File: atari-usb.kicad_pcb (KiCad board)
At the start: 2 copper layers, 30.5 x 17.8 mm, 39 parts, among them J1 USB_A, J2 DB9_Male, U1 ATmega32U4-AU, U2 TPD2EUSB30

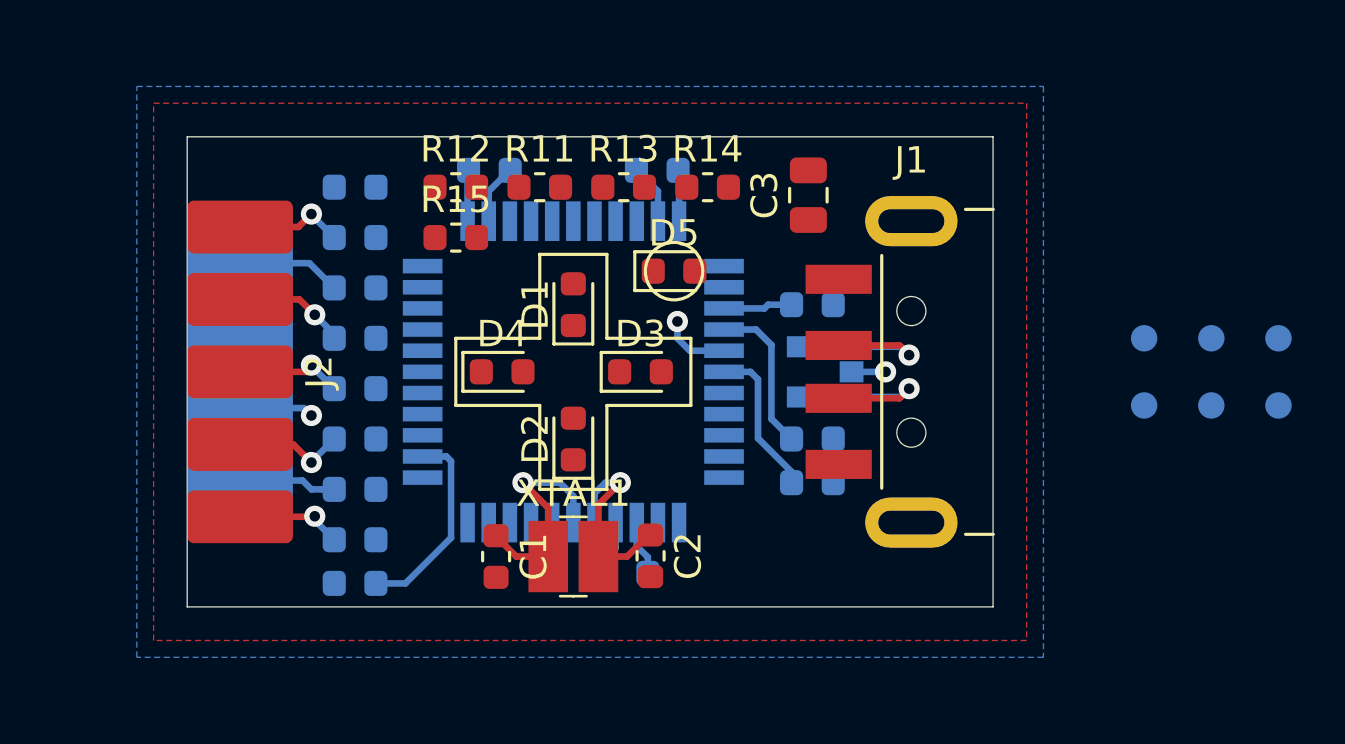
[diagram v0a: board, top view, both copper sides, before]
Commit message: Revision 0 done
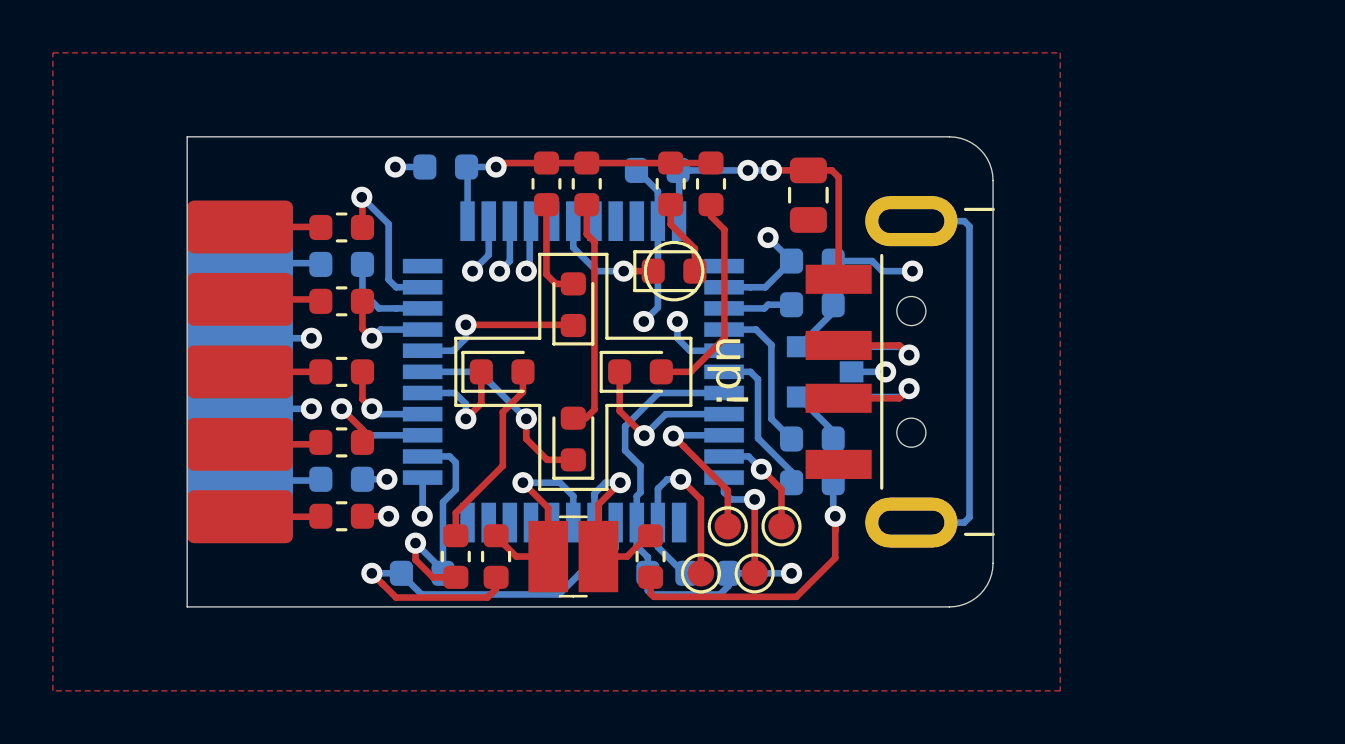
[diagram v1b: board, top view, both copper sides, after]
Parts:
- removed TP2, TP6: TestPoint, TestPoint:TestPoint_Pad_D1.0mm
- added C9: 0.1u, Capacitor_SMD:C_0603_1608Metric, B.Cu at (145.6, 80.3)
- R10, R4, R6, R7, R8: moved to F.Cu
- TP1: value TestPoint -> MISO; moved to F.Cu
- TP3: value TestPoint -> SCK; moved to F.Cu
- TP4: value TestPoint -> MOSI; moved to F.Cu
- TP5: value TestPoint -> ~RST; moved to F.Cu
- moved TP4 20.1 mm to (144.4, 90.3)
- moved R3 19.8 mm to (141.6, 92.1), turned to 180 degrees
- moved TP3 19.6 mm to (142.4, 90.3)
- moved TP5 17.9 mm to (141.4, 92.1)
- moved TP1 17.2 mm to (143.4, 92.1)
- moved R14 16.9 mm to (132.1, 91.4), turned to 90 degrees
- moved R15 8.38 mm to (140.2, 77.3), turned to 270 degrees
- moved R12 4.95 mm to (137.0, 77.3), turned to 270 degrees
- moved R13 3.30 mm to (141.7, 77.3), turned to 270 degrees
- moved C5 2.57 mm to (130.8, 92.1)
- moved C6 1.66 mm to (131.7, 76.7), turned to 0 degrees
- moved R8 1.49 mm to (127.8, 81.8)
- moved R4 1.02 mm to (127.8, 89.9)
- moved R9 1.02 mm to (127.8, 80.4)
- moved R7 0.81 mm to (127.8, 84.5)
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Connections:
- D5 pad 1: Net-(D5-Pad1) -> LED-Down
- J2 pad 7: +5V -> VBUS
- R11 pad 1: +5V -> VBUS
- R12 pad 1: +5V -> VBUS
- R13 pad 1: +5V -> VBUS
- R14 pad 1: +5V -> VBUS
- R15 pad 1: +5V -> VBUS
- R3 pad 1: +5V -> VBUS
- TP5 pad 1: Net-(TP5-Pad1) -> Net-(R3-Pad2)
- U1 pad 1: Net-(U1-Pad1) -> (no net)
- U1 pad 10: Net-(U1-Pad10) -> Net-(TP4-Pad1)
- U1 pad 11: Net-(U1-Pad11) -> Net-(TP1-Pad1)
- U1 pad 12: Net-(U1-Pad12) -> (no net)
- U1 pad 18: Net-(U1-Pad18) -> (no net)
- U1 pad 19: Net-(U1-Pad19) -> (no net)
- U1 pad 20: Net-(U1-Pad20) -> (no net)
- U1 pad 21: Net-(U1-Pad21) -> (no net)
- U1 pad 22: Net-(U1-Pad22) -> (no net)
- U1 pad 25: Net-(U1-Pad25) -> Net-(R6-Pad2)
- U1 pad 26: Net-(U1-Pad26) -> Net-(R7-Pad2)
- U1 pad 27: Net-(U1-Pad27) -> Net-(D4-Pad1)
- U1 pad 28: Net-(U1-Pad28) -> Net-(D2-Pad1)
- U1 pad 29: Net-(U1-Pad29) -> Net-(D1-Pad1)
- U1 pad 30: Net-(U1-Pad30) -> Net-(R8-Pad2)
- U1 pad 31: Net-(U1-Pad31) -> Net-(R9-Pad2)
- U1 pad 32: Net-(U1-Pad32) -> Net-(R10-Pad2)
- U1 pad 33: Net-(U1-Pad33) -> (no net)
- U1 pad 36: Net-(U1-Pad36) -> Net-(R5-Pad2)
- U1 pad 37: Net-(D5-Pad1) -> Net-(R4-Pad2)
- U1 pad 38: Net-(D4-Pad1) -> (no net)
- U1 pad 39: Net-(D3-Pad1) -> LED-Down
- U1 pad 40: Net-(D2-Pad1) -> (no net)
- U1 pad 41: Net-(D1-Pad1) -> (no net)
- U1 pad 42: Net-(U1-Pad42) -> (no net)
- U1 pad 8: Net-(U1-Pad8) -> Net-(D3-Pad1)
- U1 pad 9: Net-(U1-Pad9) -> Net-(TP3-Pad1)
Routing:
- net VBUS: track 13.6 -> 57.3 mm, vias 0 -> 7
- net GND: track 13.3 -> 49.7 mm, vias 3 -> 10
- net Net-(J1-Pad5): track 0.00 -> 15.6 mm
- net Net-(R4-Pad2): track 0.00 -> 14.4 mm, vias 0 -> 2
- net Net-(R5-Pad2): track 0.00 -> 12.6 mm, vias 0 -> 2
- net Net-(D2-Pad2): track 0.00 -> 8.78 mm
- net Net-(R3-Pad2): track 0.00 -> 8.60 mm, vias 0 -> 1
- net Net-(D3-Pad2): track 0.00 -> 8.18 mm
- net Net-(D2-Pad1): track 0.00 -> 7.52 mm, vias 0 -> 1
- net Net-(D4-Pad2): track 0.00 -> 7.25 mm
- net Net-(D1-Pad1): track 0.00 -> 6.41 mm, vias 0 -> 1
- net Net-(TP3-Pad1): track 0.00 -> 6.19 mm, vias 0 -> 1
- net Net-(D3-Pad1): track 0.00 -> 6.15 mm, vias 0 -> 1
- net Net-(R10-Pad2): track 0.00 -> 6.10 mm, vias 0 -> 1
- net Net-(R6-Pad2): track 0.00 -> 5.07 mm, vias 0 -> 1
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- added copper zone on In1.Cu, net GND
- added copper zone on In2.Cu, net VBUS
- removed copper zone on B.Cu, net GND
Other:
- outline, holes or cut-outs redrawn
- copper layers 2 -> 4
- board text added: "GH: jomag"
- board text added: "atari usb"
- board text added: "rev 0"
- board text added: "up!"
